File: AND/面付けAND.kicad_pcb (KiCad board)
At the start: 2 copper layers, 99.9 x 53.4 mm, 90 parts

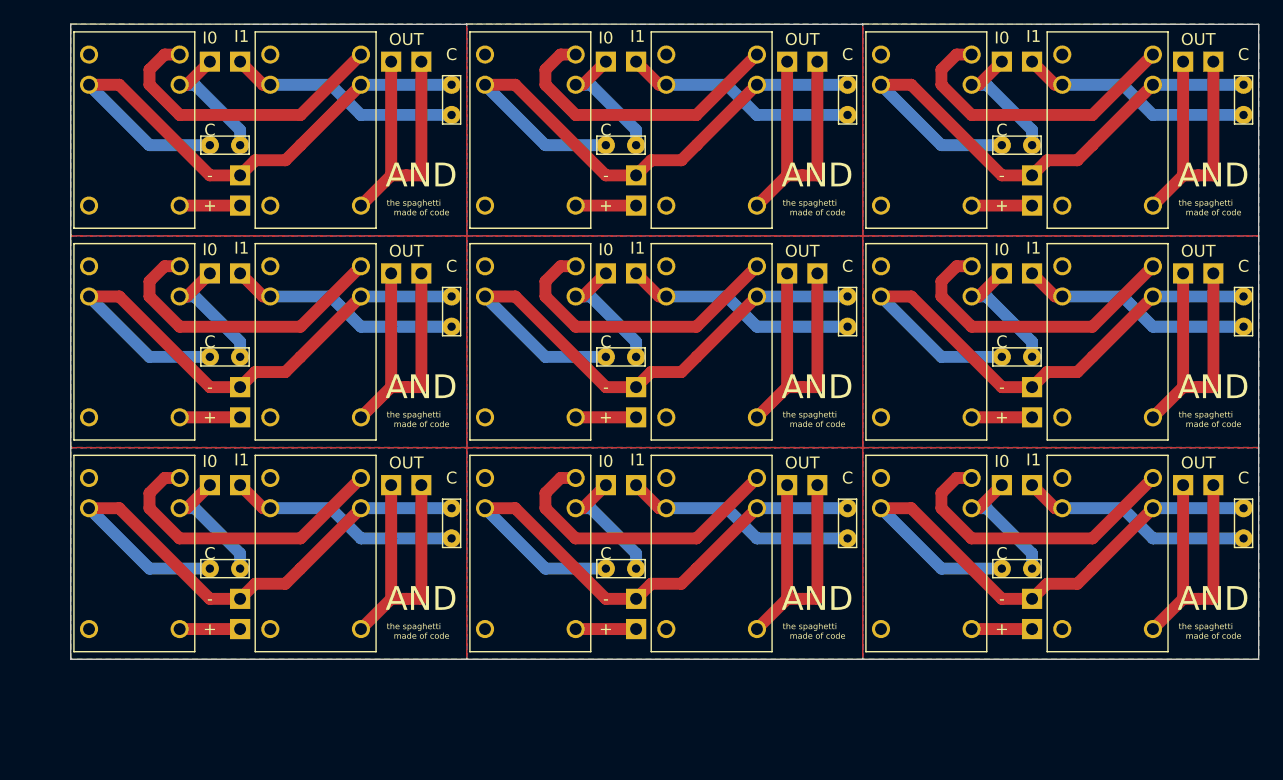
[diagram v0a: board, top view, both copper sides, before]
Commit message: Add files via upload
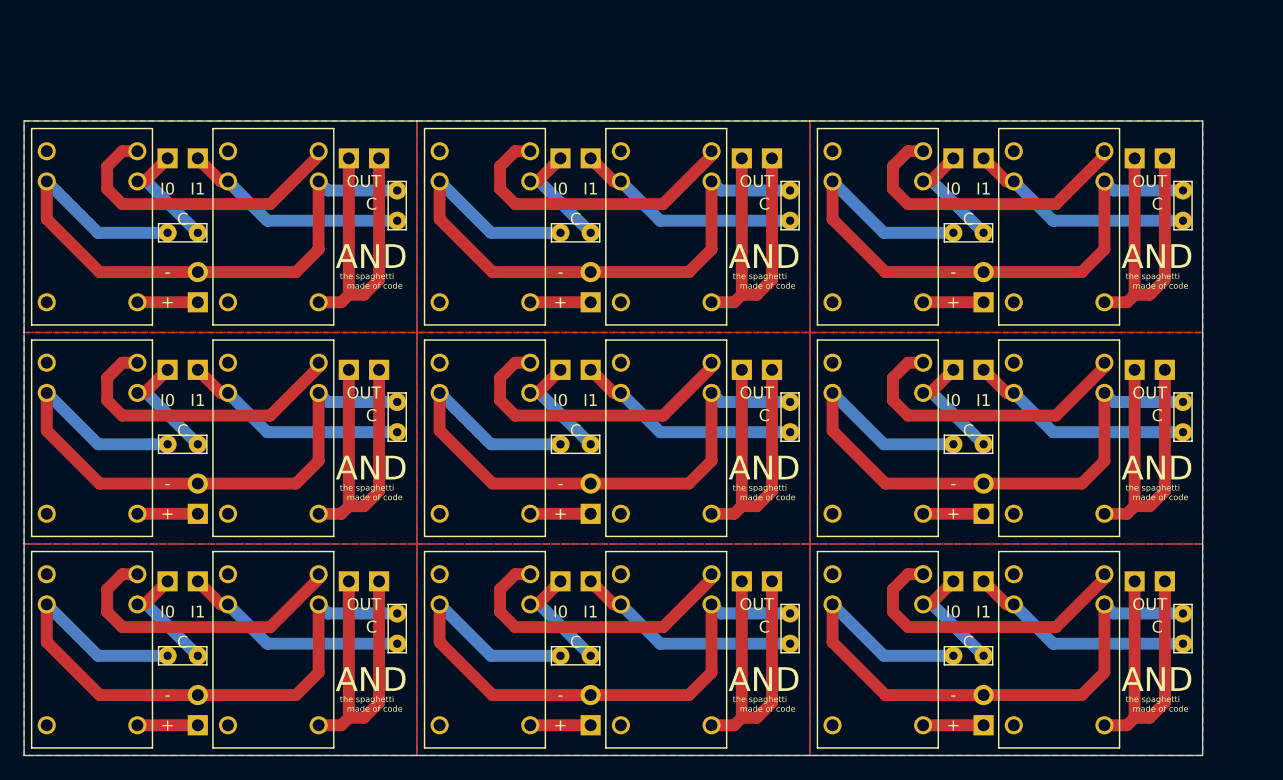
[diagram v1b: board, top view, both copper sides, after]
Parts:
- removed REF** (x54): PinHeader_1x01_P2.54mm_Vertical, Connector_PinHeader_2.54mm:PinHeader_1x01_P2.54mm_Vertical
- removed REF** (x18): 946H-1C-24D, MiyakeFootprintLib:946H-1C-24D
- removed REF** (x18): Condensor, MiyakeFootprintLib:Condensor
- added C1: C, MiyakeFootprintLib:Condensor, F.Cu at (135.9, 93.2)
- added C1: C, MiyakeFootprintLib:Condensor, F.Cu at (102.9, 93.2)
- added C1: C, MiyakeFootprintLib:Condensor, F.Cu at (69.8, 93.2)
- added C1: C, MiyakeFootprintLib:Condensor, F.Cu at (135.9, 75.4)
- added C1: C, MiyakeFootprintLib:Condensor, F.Cu at (102.9, 75.4)
- added C1: C, MiyakeFootprintLib:Condensor, F.Cu at (69.8, 75.4)
- added C1: C, MiyakeFootprintLib:Condensor, F.Cu at (135.9, 57.7)
- added C1: C, MiyakeFootprintLib:Condensor, F.Cu at (102.9, 57.7)
- added C1: C, MiyakeFootprintLib:Condensor, F.Cu at (69.8, 57.7)
- added C2: C, MiyakeFootprintLib:Condensor, F.Cu at (152.7, 89.7)
- added C2: C, MiyakeFootprintLib:Condensor, F.Cu at (119.6, 89.7)
- added C2: C, MiyakeFootprintLib:Condensor, F.Cu at (86.6, 89.7)
- added C2: C, MiyakeFootprintLib:Condensor, F.Cu at (152.7, 71.9)
- added C2: C, MiyakeFootprintLib:Condensor, F.Cu at (119.6, 71.9)
- added C2: C, MiyakeFootprintLib:Condensor, F.Cu at (86.6, 71.9)
- added C2: C, MiyakeFootprintLib:Condensor, F.Cu at (152.7, 54.1)
- added C2: C, MiyakeFootprintLib:Condensor, F.Cu at (119.6, 54.1)
- added C2: C, MiyakeFootprintLib:Condensor, F.Cu at (86.6, 54.1)
- added J1: Conn_01x01, Connector_PinHeader_2.54mm:PinHeader_1x01_P2.54mm_Vertical, B.Cu at (133.4, 87.0)
- added J1: Conn_01x01, Connector_PinHeader_2.54mm:PinHeader_1x01_P2.54mm_Vertical, B.Cu at (100.3, 87.0)
- added J1: Conn_01x01, Connector_PinHeader_2.54mm:PinHeader_1x01_P2.54mm_Vertical, B.Cu at (67.3, 87.0)
- added J1: Conn_01x01, Connector_PinHeader_2.54mm:PinHeader_1x01_P2.54mm_Vertical, B.Cu at (133.4, 69.2)
- added J1: Conn_01x01, Connector_PinHeader_2.54mm:PinHeader_1x01_P2.54mm_Vertical, B.Cu at (100.3, 69.2)
- added J1: Conn_01x01, Connector_PinHeader_2.54mm:PinHeader_1x01_P2.54mm_Vertical, B.Cu at (67.3, 69.2)
- added J1: Conn_01x01, Connector_PinHeader_2.54mm:PinHeader_1x01_P2.54mm_Vertical, B.Cu at (133.4, 51.4)
- added J1: Conn_01x01, Connector_PinHeader_2.54mm:PinHeader_1x01_P2.54mm_Vertical, B.Cu at (100.3, 51.4)
- added J1: Conn_01x01, Connector_PinHeader_2.54mm:PinHeader_1x01_P2.54mm_Vertical, B.Cu at (67.3, 51.4)
- added J2: Conn_01x01, Connector_PinHeader_2.54mm:PinHeader_1x01_P2.54mm_Vertical, B.Cu at (135.9, 87.0)
- added J2: Conn_01x01, Connector_PinHeader_2.54mm:PinHeader_1x01_P2.54mm_Vertical, B.Cu at (102.9, 87.0)
- added J2: Conn_01x01, Connector_PinHeader_2.54mm:PinHeader_1x01_P2.54mm_Vertical, B.Cu at (69.8, 87.0)
- added J2: Conn_01x01, Connector_PinHeader_2.54mm:PinHeader_1x01_P2.54mm_Vertical, B.Cu at (135.9, 69.2)
- added J2: Conn_01x01, Connector_PinHeader_2.54mm:PinHeader_1x01_P2.54mm_Vertical, B.Cu at (102.9, 69.2)
- added J2: Conn_01x01, Connector_PinHeader_2.54mm:PinHeader_1x01_P2.54mm_Vertical, B.Cu at (69.8, 69.2)
- added J2: Conn_01x01, Connector_PinHeader_2.54mm:PinHeader_1x01_P2.54mm_Vertical, B.Cu at (135.9, 51.4)
- added J2: Conn_01x01, Connector_PinHeader_2.54mm:PinHeader_1x01_P2.54mm_Vertical, B.Cu at (102.9, 51.4)
- added J2: Conn_01x01, Connector_PinHeader_2.54mm:PinHeader_1x01_P2.54mm_Vertical, B.Cu at (69.8, 51.4)
- added J3: Conn_01x01, Connector_PinHeader_2.54mm:PinHeader_1x01_P2.54mm_Vertical, B.Cu at (148.6, 87.0)
- added J3: Conn_01x01, Connector_PinHeader_2.54mm:PinHeader_1x01_P2.54mm_Vertical, B.Cu at (115.6, 87.0)
- added J3: Conn_01x01, Connector_PinHeader_2.54mm:PinHeader_1x01_P2.54mm_Vertical, B.Cu at (82.5, 87.0)
- added J3: Conn_01x01, Connector_PinHeader_2.54mm:PinHeader_1x01_P2.54mm_Vertical, B.Cu at (148.6, 69.2)
- added J3: Conn_01x01, Connector_PinHeader_2.54mm:PinHeader_1x01_P2.54mm_Vertical, B.Cu at (115.6, 69.2)
- added J3: Conn_01x01, Connector_PinHeader_2.54mm:PinHeader_1x01_P2.54mm_Vertical, B.Cu at (82.5, 69.2)
- added J3: Conn_01x01, Connector_PinHeader_2.54mm:PinHeader_1x01_P2.54mm_Vertical, B.Cu at (148.6, 51.4)
- added J3: Conn_01x01, Connector_PinHeader_2.54mm:PinHeader_1x01_P2.54mm_Vertical, B.Cu at (115.6, 51.4)
- added J3: Conn_01x01, Connector_PinHeader_2.54mm:PinHeader_1x01_P2.54mm_Vertical, B.Cu at (82.5, 51.4)
- added J4: Conn_01x01, Connector_PinHeader_2.54mm:PinHeader_1x01_P2.54mm_Vertical, B.Cu at (151.2, 87.0)
- added J4: Conn_01x01, Connector_PinHeader_2.54mm:PinHeader_1x01_P2.54mm_Vertical, B.Cu at (118.1, 87.0)
- added J4: Conn_01x01, Connector_PinHeader_2.54mm:PinHeader_1x01_P2.54mm_Vertical, B.Cu at (85.1, 87.0)
- added J4: Conn_01x01, Connector_PinHeader_2.54mm:PinHeader_1x01_P2.54mm_Vertical, B.Cu at (151.2, 69.2)
- added J4: Conn_01x01, Connector_PinHeader_2.54mm:PinHeader_1x01_P2.54mm_Vertical, B.Cu at (118.1, 69.2)
- added J4: Conn_01x01, Connector_PinHeader_2.54mm:PinHeader_1x01_P2.54mm_Vertical, B.Cu at (85.1, 69.2)
- added J4: Conn_01x01, Connector_PinHeader_2.54mm:PinHeader_1x01_P2.54mm_Vertical, B.Cu at (151.2, 51.4)
- added J4: Conn_01x01, Connector_PinHeader_2.54mm:PinHeader_1x01_P2.54mm_Vertical, B.Cu at (118.1, 51.4)
- added J4: Conn_01x01, Connector_PinHeader_2.54mm:PinHeader_1x01_P2.54mm_Vertical, B.Cu at (85.1, 51.4)
- added J5: Conn_01x02, Connector_PinHeader_2.54mm:PinHeader_1x02_P2.54mm_Vertical, B.Cu at (135.9, 99.1)
- added J5: Conn_01x02, Connector_PinHeader_2.54mm:PinHeader_1x02_P2.54mm_Vertical, B.Cu at (102.9, 99.1)
- added J5: Conn_01x02, Connector_PinHeader_2.54mm:PinHeader_1x02_P2.54mm_Vertical, B.Cu at (69.8, 99.1)
- added J5: Conn_01x02, Connector_PinHeader_2.54mm:PinHeader_1x02_P2.54mm_Vertical, B.Cu at (135.9, 81.3)
- added J5: Conn_01x02, Connector_PinHeader_2.54mm:PinHeader_1x02_P2.54mm_Vertical, B.Cu at (102.9, 81.3)
- added J5: Conn_01x02, Connector_PinHeader_2.54mm:PinHeader_1x02_P2.54mm_Vertical, B.Cu at (69.8, 81.3)
- added J5: Conn_01x02, Connector_PinHeader_2.54mm:PinHeader_1x02_P2.54mm_Vertical, B.Cu at (135.9, 63.5)
- added J5: Conn_01x02, Connector_PinHeader_2.54mm:PinHeader_1x02_P2.54mm_Vertical, B.Cu at (102.9, 63.5)
- added J5: Conn_01x02, Connector_PinHeader_2.54mm:PinHeader_1x02_P2.54mm_Vertical, B.Cu at (69.8, 63.5)
- added SPDT1: 946H-1C-24D, MiyakeFootprintLib:946H-1C-24D, F.Cu at (128.3, 91.4)
- added SPDT1: 946H-1C-24D, MiyakeFootprintLib:946H-1C-24D, F.Cu at (95.3, 91.4)
- added SPDT1: 946H-1C-24D, MiyakeFootprintLib:946H-1C-24D, F.Cu at (62.2, 91.4)
- added SPDT1: 946H-1C-24D, MiyakeFootprintLib:946H-1C-24D, F.Cu at (128.3, 73.7)
- added SPDT1: 946H-1C-24D, MiyakeFootprintLib:946H-1C-24D, F.Cu at (95.3, 73.7)
- added SPDT1: 946H-1C-24D, MiyakeFootprintLib:946H-1C-24D, F.Cu at (62.2, 73.7)
- added SPDT1: 946H-1C-24D, MiyakeFootprintLib:946H-1C-24D, F.Cu at (128.3, 55.9)
- added SPDT1: 946H-1C-24D, MiyakeFootprintLib:946H-1C-24D, F.Cu at (95.3, 55.9)
- added SPDT1: 946H-1C-24D, MiyakeFootprintLib:946H-1C-24D, F.Cu at (62.2, 55.9)
- added SPDT2: 946H-1C-24D, MiyakeFootprintLib:946H-1C-24D, F.Cu at (143.5, 91.4)
- added SPDT2: 946H-1C-24D, MiyakeFootprintLib:946H-1C-24D, F.Cu at (110.5, 91.4)
- added SPDT2: 946H-1C-24D, MiyakeFootprintLib:946H-1C-24D, F.Cu at (77.5, 91.4)
- added SPDT2: 946H-1C-24D, MiyakeFootprintLib:946H-1C-24D, F.Cu at (143.5, 73.7)
- added SPDT2: 946H-1C-24D, MiyakeFootprintLib:946H-1C-24D, F.Cu at (110.5, 73.7)
- added SPDT2: 946H-1C-24D, MiyakeFootprintLib:946H-1C-24D, F.Cu at (77.5, 73.7)
- added SPDT2: 946H-1C-24D, MiyakeFootprintLib:946H-1C-24D, F.Cu at (143.5, 55.9)
- added SPDT2: 946H-1C-24D, MiyakeFootprintLib:946H-1C-24D, F.Cu at (110.5, 55.9)
- added SPDT2: 946H-1C-24D, MiyakeFootprintLib:946H-1C-24D, F.Cu at (77.5, 55.9)
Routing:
- net (no net): track 1220.1 -> 0.00 mm
- net GND: track 0.00 -> 479.2 mm
- net +24V: track 0.00 -> 273.8 mm
- net Net-(J3-Pad1): track 0.00 -> 247.8 mm
- net Net-(C2-Pad2): track 0.00 -> 170.4 mm
- net Net-(C1-Pad1): track 0.00 -> 91.9 mm
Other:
- board size 99.9 x 53.4 mm -> 99.1 x 53.3 mm
- board text removed: "V-CUT"
